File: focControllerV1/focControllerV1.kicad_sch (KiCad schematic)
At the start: 40 parts, among them SW1 SW_Push, U1 LP2992IM5X-5.0/NOPB, U2 ME3116AM6G, U3 STM32F103C8Tx, Y1 Crystal_GND2_Small

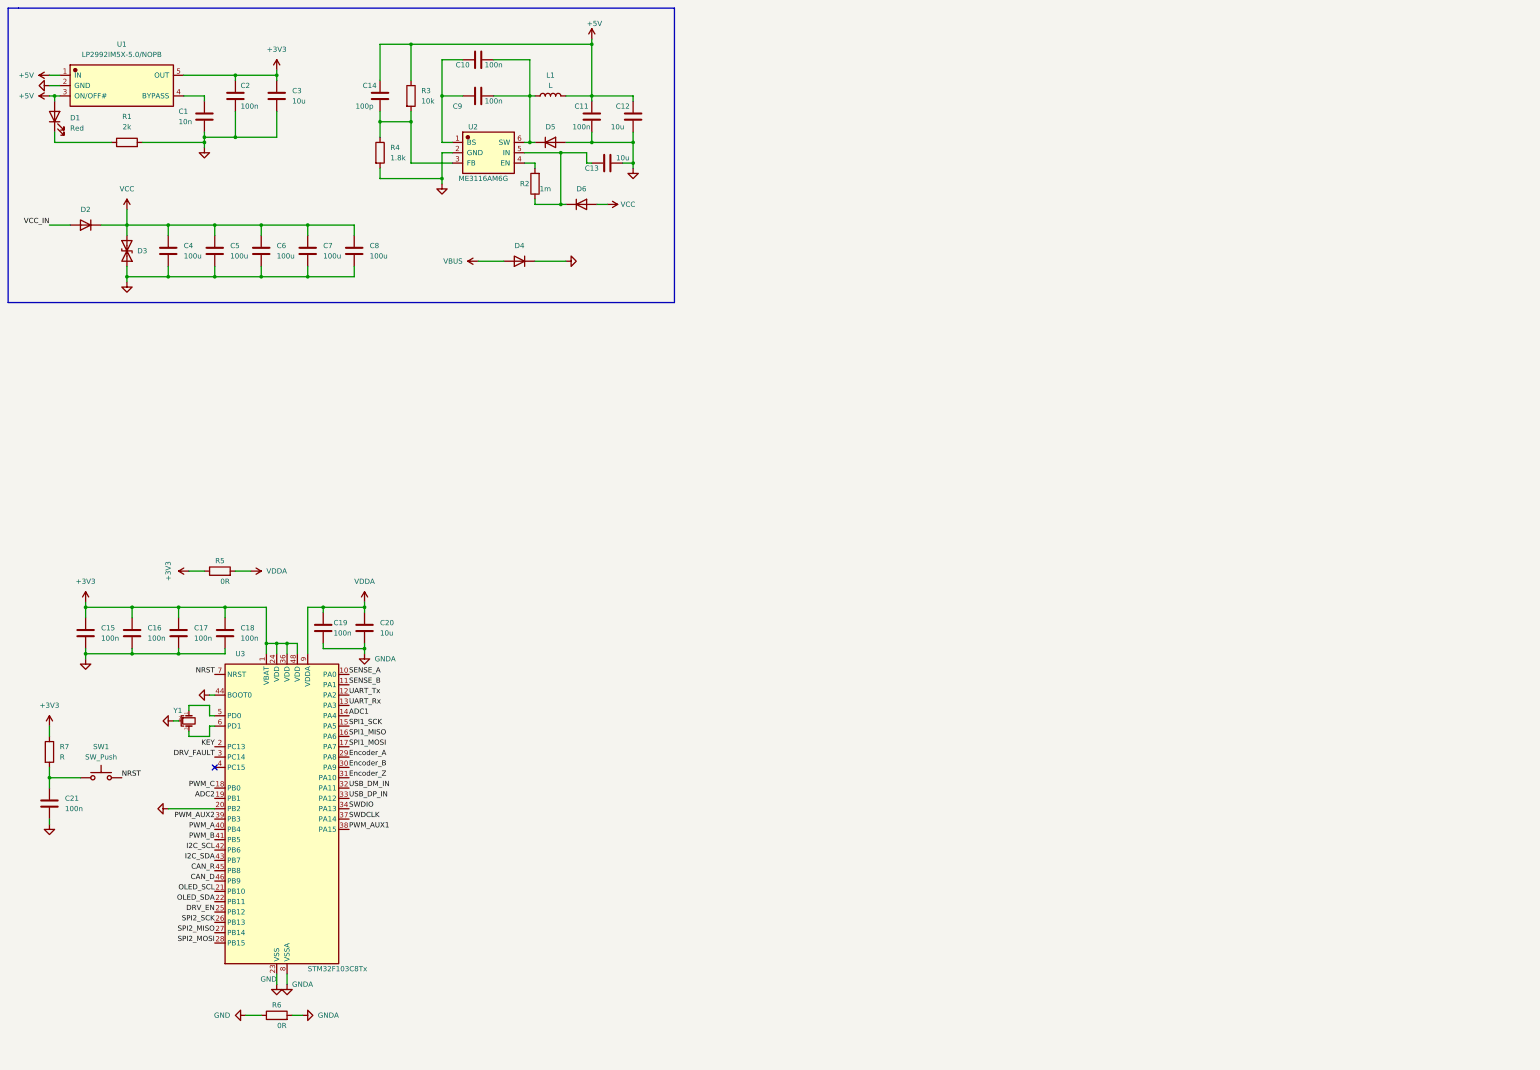
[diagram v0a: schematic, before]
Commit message: 原理图设计中
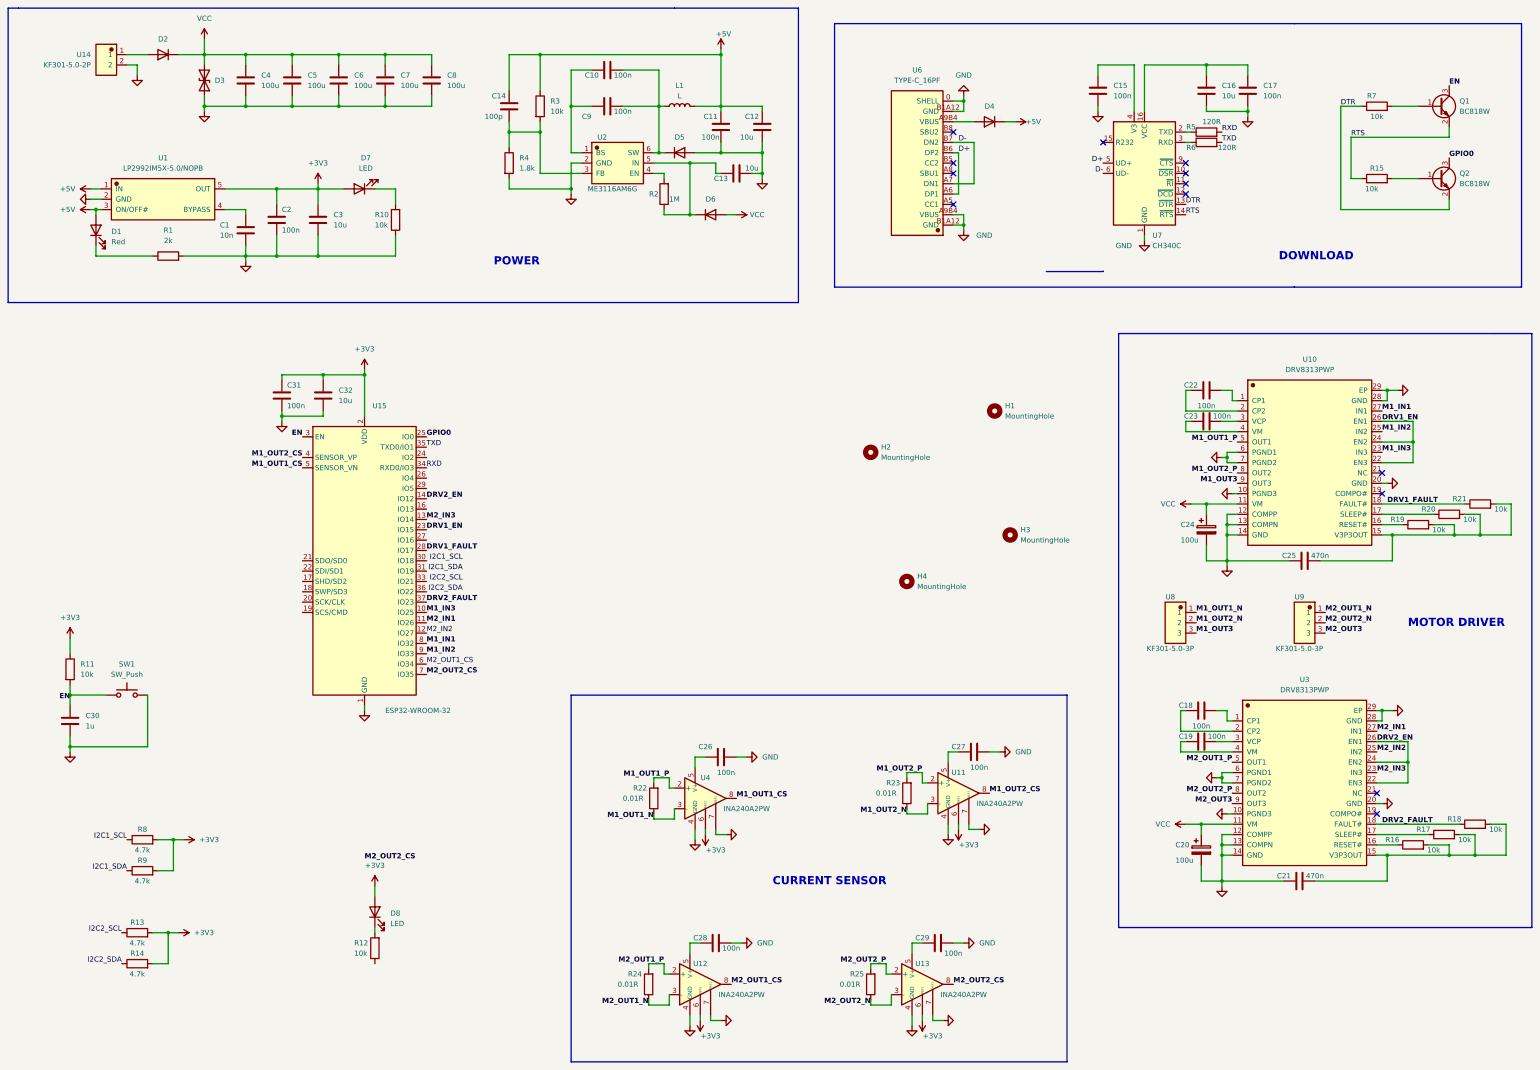
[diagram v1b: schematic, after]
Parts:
- removed C20: 10u, symbol Device:C
- removed U3: STM32F103C8Tx, Package_QFP:LQFP-48_7x7mm_P0.5mm, symbol MCU_ST_STM32F1:STM32F103C8Tx
- removed Y1: Crystal_GND2_Small, symbol Device:Crystal_GND2_Small
- added C20, C24: 100u, symbol Device:C_Polarized
- added C22, C23, C26, C27, C28, C29, C31: 100n, symbol Device:C
- added C25: 470n, symbol Device:C
- added C30: 1u, symbol Device:C
- added C32: 10u, symbol Device:C
- added D7, D8: LED, symbol Device:LED
- added H1, H2, H3, H4: MountingHole, symbol Mechanical:MountingHole
- added Q1, Q2: BC818W, Package_TO_SOT_SMD:SOT-323_SC-70, symbol Transistor_BJT:BC818W
- added R10, R11, R12, R15, R16, R17, R18, R19, R20, R21: 10k, symbol Device:R
- added R13, R14, R8, R9: 4.7k, symbol Device:R
- added R22, R23, R24, R25: 0.01R, symbol Device:R
- added U10, U3: DRV8313PWP, kicad_lceda:TSSOP-28_L9.7-W4.4-P0.65-LS6.4-TL-EP-2, symbol duanpu:DRV8313PWP
- added U11, U12, U13, U4: INA240A2PW, Package_SO:TSSOP-8_4.4x3mm_P0.65mm, symbol Amplifier_Current:INA240A2PW
- added U14: KF301-5.0-2P, kicad_lceda:CONN-TH_P5.00_KF301-5.0-2P, symbol duanpu:KF301-5.0-2P
- added U15: ESP32-WROOM-32, RF_Module:ESP32-WROOM-32, symbol RF_Module:ESP32-WROOM-32
- added U6: TYPE-C_16PF, kicad_lceda:USB-C-SMD_TYPE-C-USB-5, symbol duanpu:TYPE-C_16PF
- added U7: CH340C, Package_SO:SOIC-16_3.9x9.9mm_P1.27mm, symbol Interface_USB:CH340C
- added U8, U9: KF301-5.0-3P, kicad_lceda:CONN-TH_3P-P5.00_KF301-5.0-3P, symbol duanpu:KF301-5.0-3P
- C16: value 100n -> 10u
- C21: value 100n -> 470n
- R2: value 1m -> 1M
- R5, R6: value 0R -> 120R
- R7: value R -> 10k
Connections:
- net NRST is gone; now on net GND: SW1.2
- net +3V3: now also C31.1, C32.1, D7.2 (A), D8.2 (A), R11.1, R13.2, R14.2, R8.2, R9.2, U11.6 (REF2), U12.6 (REF2), U13.6 (REF2), U15.2 (VDD), U4.6 (REF2); no longer C15.2, C16.2, C17.2, C18.2, R5.1, R7.1
- net +5V: now also D4.1 (K)
- net GND: now also C15.2, C16.2, C17.2, C20.2, C24.2, C25.1, C26.2, C27.2, C28.2, C29.2, C30.2, C31.2, C32.2, R10.1, U10.10 (PGND3), U10.12 (COMPP), U10.13 (COMPN), U10.14 (GND), U10.20 (GND), U10.28 (GND), U10.29 (EP), U10.6 (PGND1), U10.7 (PGND2), U11.1 (GND), U11.4 (GND), U11.7 (REF1), U12.1 (GND), U12.4 (GND), U12.7 (REF1), U13.1 (GND), U13.4 (GND), U13.7 (REF1), U14.2, U15.1 (GND), U15.15 (GND), U15.38 (GND), U15.39 (GND), U3.10 (PGND3), U3.12 (COMPP), U3.13 (COMPN), U3.14 (GND), U3.20 (GND), U3.28 (GND), U3.29 (EP), U3.6 (PGND1), U3.7 (PGND2), U4.1 (GND), U4.4 (GND), U4.7 (REF1), U6.0 (SHELL), U6.A9B4 (VBUS), U6.B1A12 (GND), U7.1 (GND); no longer C15.1, C16.1, C17.1, C18.1, D4.1 (K), R6.1
- net VCC: now also C20.1, C24.1, U10.11 (VM), U3.11 (VM)
- net GNDA: no longer names the net of C19.2
- net GNDA: now also U3.3 (VCP); no longer R6.2
- net VBUS: no longer names the net of D4.2 (A)
- net VBUS: now also U6.A9B4 (VBUS)
- net VCC_IN: no longer names the net of D2.2 (A)
- net VCC_IN: now also U14.1
- net VDDA: no longer names the net of C19.1
- net VDDA: now also U3.4 (VM); no longer R5.2
- new net: C16.1, C17.1, U7.16 (VCC)
- new net: Q2.1 (B), R15.2
- new net: C26.1, U4.5 (V+)
- new net: D7.1 (K), R10.2
- new net: C18.2, U3.1 (CP1)
- new net: C21.2, R16.2, R17.2, R18.2, U3.15 (V3P3OUT)
- new net: R16.1, U3.16 (RESET#)
- new net: R17.1, U3.17 (SLEEP#)
- new net: C18.1, U3.2 (CP2)
- new net: C28.1, U12.5 (V+)
- new net: C29.1, U13.5 (V+)
- new net: Q1.1 (B), R7.2
- new net: C27.1, U11.5 (V+)
- new net: R5.1, U7.2 (TXD)
- new net: R6.1, U7.3 (RXD)
- new net: C15.1, U7.4 (V3)
- new net: C25.2, R19.2, R20.2, R21.2, U10.15 (V3P3OUT)
- new net: R19.1, U10.16 (RESET#)
- new net: C23.1, U10.4 (VM)
- new net: C23.2, U10.3 (VCP)
- new net: C22.1, U10.2 (CP2)
- new net: C22.2, U10.1 (CP1)
- new net: D8.1 (K), R12.2
- new net: R20.1, U10.17 (SLEEP#)
- new net D+: U6.A6 (DP1), U6.B6 (DP2), U7.5 (UD+)
- new net D-: U6.A7 (DN1), U6.B7 (DN2), U7.6 (UD-)
- new net DRV1_EN: U10.22 (EN3), U10.24 (EN2), U10.26 (EN1), U15.23 (IO15)
- new net DRV1_FAULT: R21.1, U10.18 (FAULT#), U15.28 (IO17)
- new net DRV2_EN: U15.14 (IO12), U3.22 (EN3), U3.24 (EN2), U3.26 (EN1)
- new net DRV2_FAULT: R18.1, U15.37 (IO23), U3.18 (FAULT#)
- new net DTR: Q2.2 (E), R7.1, U7.13 (~{DTR})
- new net EN: C30.1, Q1.3 (C), R11.2, SW1.1, U15.3 (EN)
- new net GPIO0: Q2.3 (C), U15.25 (IO0)
- new net I2C1_SCL: R8.1
- new net I2C1_SDA: R9.1
- new net I2C2_SCL: R13.1
- new net I2C2_SDA: R14.1
- new net M1_IN1: U10.27 (IN1), U15.8 (IO32)
- new net M1_IN2: U10.25 (IN2), U15.9 (IO33)
- new net M1_IN3: U10.23 (IN3), U15.10 (IO25)
- new net M1_OUT1_CS: U15.5 (SENSOR_VN), U4.8
- new net M1_OUT1_N: R22.1, U4.3 (-), U8.1
- new net M1_OUT1_P: R22.2, U10.5 (OUT1), U4.2 (+)
- new net M1_OUT2_CS: U11.8, U15.4 (SENSOR_VP)
- new net M1_OUT2_N: R23.1, U11.3 (-), U8.2
- new net M1_OUT2_P: R23.2, U10.8 (OUT2), U11.2 (+)
- new net M1_OUT3: U10.9 (OUT3), U8.3
- new net M2_IN1: U15.11 (IO26), U3.27 (IN1)
- new net M2_IN2: U15.12 (IO27), U3.25 (IN2)
- new net M2_IN3: U15.13 (IO14), U3.23 (IN3)
- new net M2_OUT1_CS: U12.8, U15.6 (IO34)
- new net M2_OUT1_N: R24.1, U12.3 (-), U9.1
- new net M2_OUT1_P: R24.2, U12.2 (+), U3.5 (OUT1)
- new net M2_OUT2_CS: U13.8, U15.7 (IO35)
- new net M2_OUT2_N: R25.1, U13.3 (-), U9.2
- new net M2_OUT2_P: R25.2, U13.2 (+), U3.8 (OUT2)
- new net M2_OUT3: U3.9 (OUT3), U9.3
- new net RTS: Q1.2 (E), R15.1, U7.14 (~{RTS})
- new net RXD: R5.2, U15.34 (RXD0/IO3)
- new net TXD: R6.2, U15.35 (TXD0/IO1)
- no-connect marks 1 -> 13
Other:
- note added: "CURRENT SENSOR"
- note added: "DOWNLOAD"
- note added: "MOTOR DRIVER"
- note added: "POWER"
- moved on the sheet: C1, C10, C11, C12, C13, C14, C2, C3, C4, C5, C6, C7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
